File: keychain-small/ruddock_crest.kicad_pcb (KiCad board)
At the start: 2 copper layers, 1 part

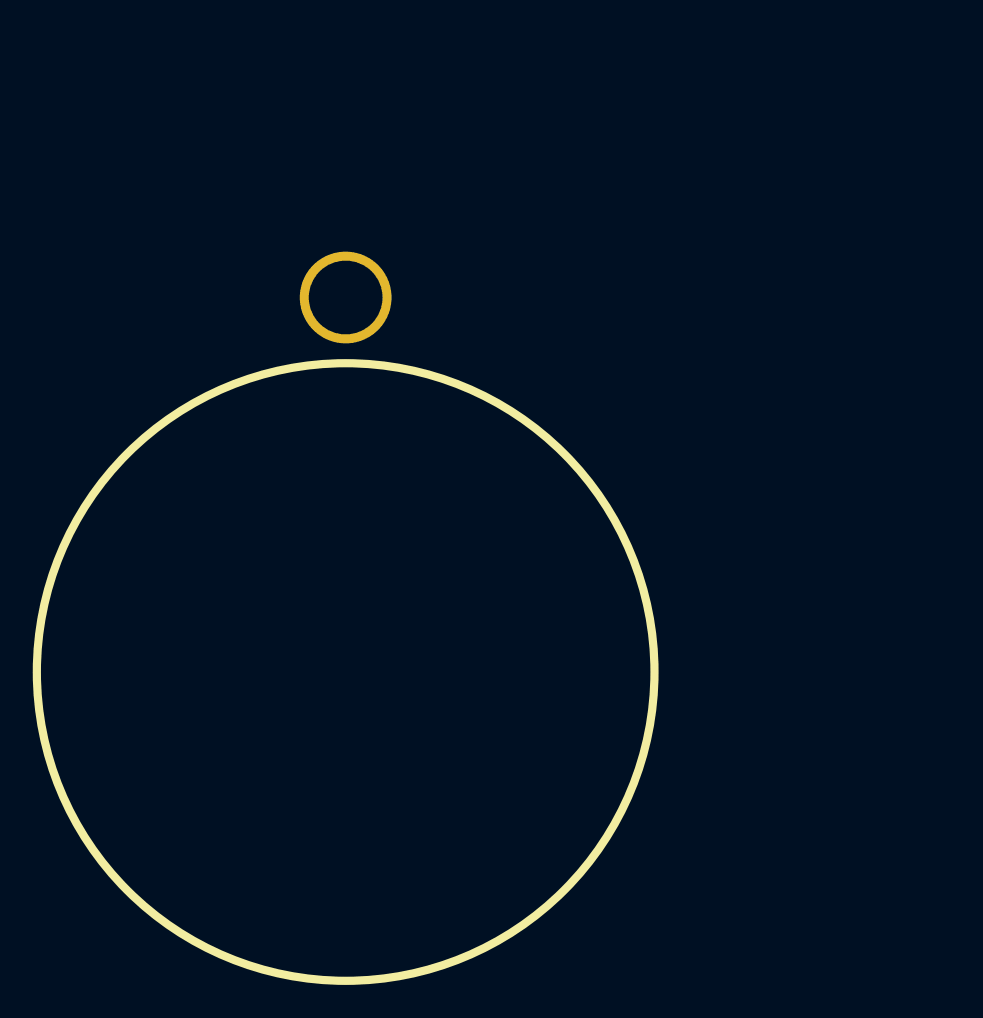
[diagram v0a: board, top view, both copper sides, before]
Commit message: Finish new design
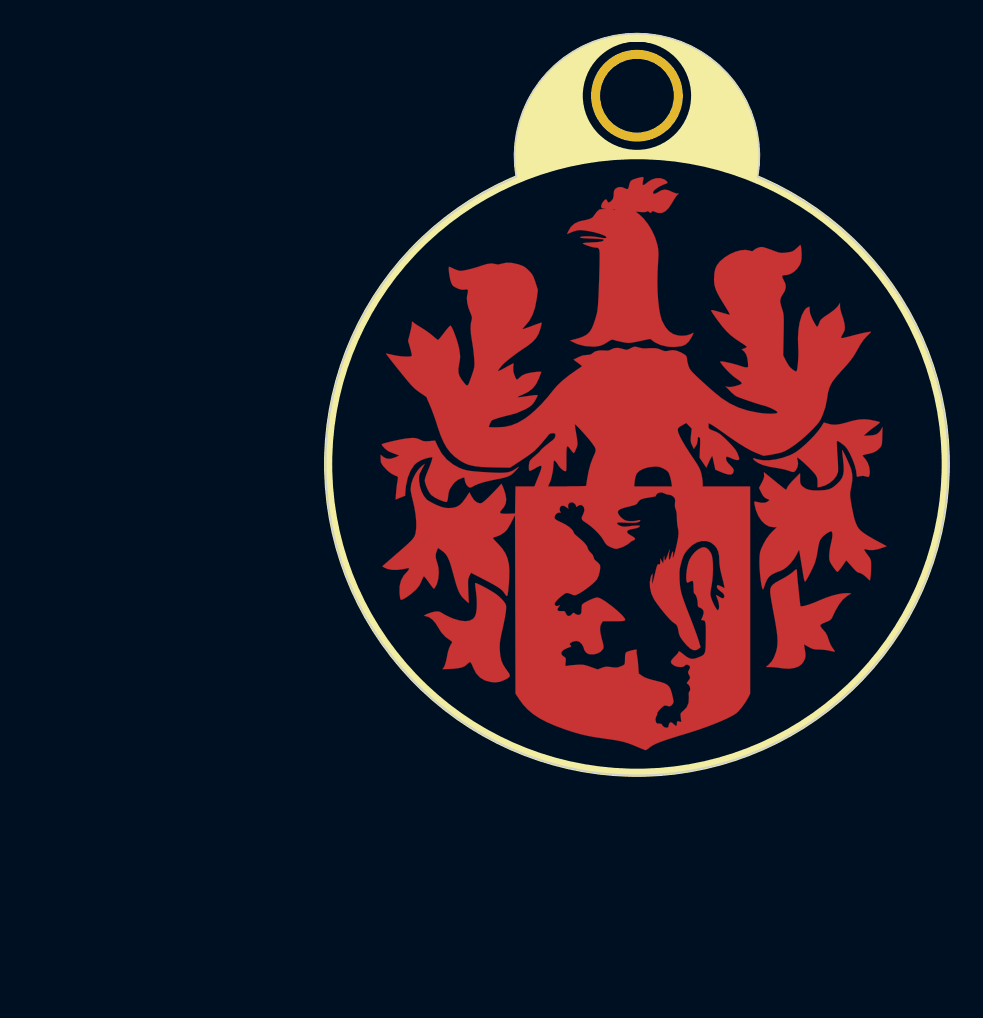
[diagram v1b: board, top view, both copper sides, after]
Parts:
- added G***: LOGO, crest:ruddock_cu_1in5, F.Cu at (141.0, 108.2)
- added G***: LOGO, crest:ruddock_fsilk_1in5, B.Cu at (141.0, 108.2)
- added G***: LOGO, crest:ruddock_mask_1in5, F.Cu at (141.0, 108.2)
- moved REF** 21.6 mm to (141.0, 85.5)
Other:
- board outline added: 38 x 45.3 mm
